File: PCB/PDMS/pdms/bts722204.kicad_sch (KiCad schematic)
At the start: 21 parts, among them IC7 BTS722204ESAXUMA1

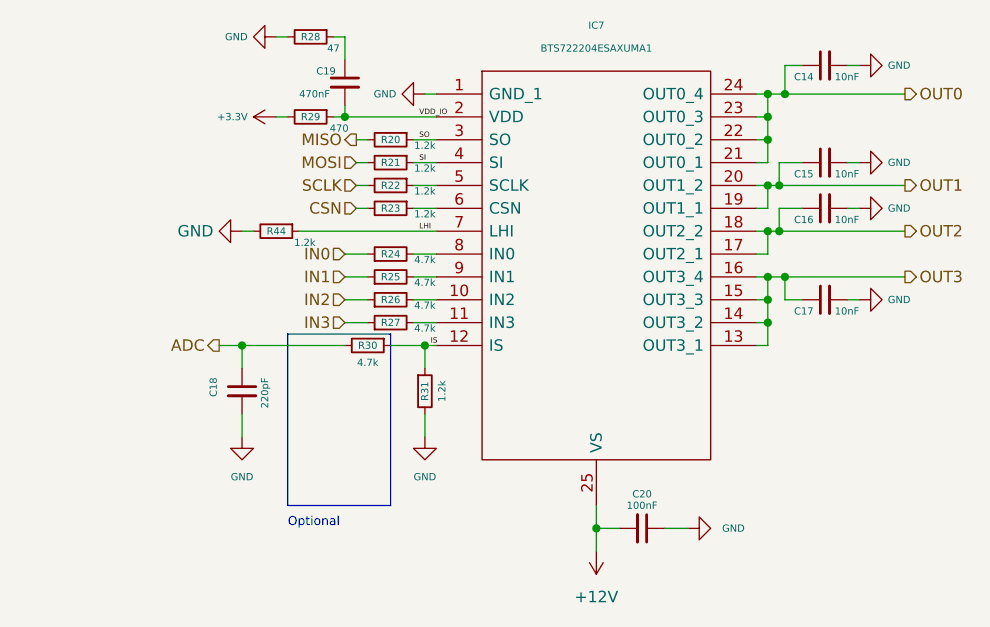
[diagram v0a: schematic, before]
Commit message: Major changes with new switch
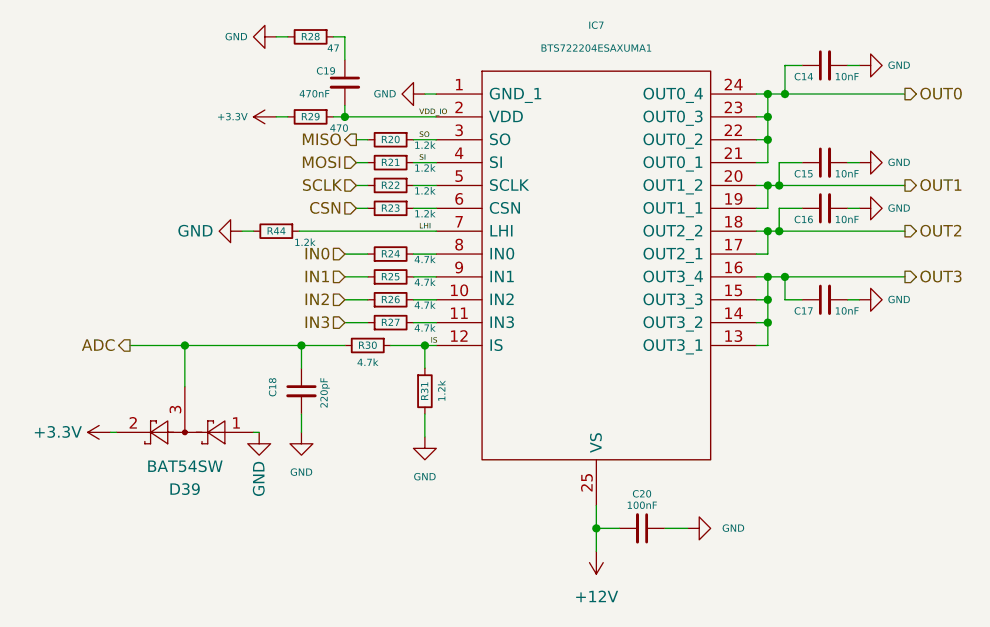
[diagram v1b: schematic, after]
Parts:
- added D39: BAT54SW, Package_TO_SOT_SMD:SOT-323_SC-70, symbol Diode:BAT54SW
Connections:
- net +3.3V: now also D39.2
- net ADC: now also D39.3
- net GND: now also D39.1
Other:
- note removed: "Optional"
- moved on the sheet: C18
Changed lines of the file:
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@@
   (junction (at 59.69 71.12) (diameter 0) (color 0 0 0 0)
   )
+  (junction (at 33.02 71.12) (diameter 0) (color 0 0 0 0)
+  )
   (junction (at 97.79 43.18) (diameter 0) (color 0 0 0 0)
   )
@@
   (junction (at 99.06 58.42) (diameter 0) (color 0 0 0 0)
   )
-  (junction (at 39.37 71.12) (diameter 0) (color 0 0 0 0)
+  (junction (at 45.974 71.12) (diameter 0) (color 0 0 0 0)
   )
   (junction (at 97.79 48.26) (diameter 0) (color 0 0 0 0)
@@
     (stroke (width 0) (type default) (color 0 0 0 0))
   )
-  (wire (pts (xy 39.37 71.12) (xy 50.8 71.12))
+  (wire (pts (xy 45.974 71.12) (xy 50.8 71.12))
     (stroke (width 0) (type default) (color 0 0 0 0))
   )
@@
     (stroke (width 0) (type default) (color 0 0 0 0))
   )
-  (polyline (pts (xy 44.45 69.85) (xy 44.45 88.9))
-    (stroke (width 0) (type default) (color 0 0 0 0))
-  )
   (wire (pts (xy 97.79 66.04) (xy 97.79 68.58))
     (stroke (width 0) (type default) (color 0 0 0 0))
@@
     (stroke (width 0) (type default) (color 0 0 0 0))
   )
-  (polyline (pts (xy 44.45 69.85) (xy 55.88 69.85))
-    (stroke (width 0) (type default) (color 0 0 0 0))
-  )
   (wire (pts (xy 50.8 66.04) (xy 53.34 66.04))
     (stroke (width 0) (type default) (color 0 0 0 0))
@@
     (stroke (width 0) (type default) (color 0 0 0 0))
   )
-  (wire (pts (xy 39.37 71.12) (xy 39.37 73.66))
+  (wire (pts (xy 45.974 71.12) (xy 45.974 73.66))
     (stroke (width 0) (type default) (color 0 0 0 0))
   )
@@
     (stroke (width 0) (type default) (color 0 0 0 0))
   )
+  (wire (pts (xy 41.275 80.772) (xy 40.64 80.772))
+    (stroke (width 0) (type default) (color 0 0 0 0))
+  )
   (wire (pts (xy 50.8 60.96) (xy 53.34 60.96))
     (stroke (width 0) (type default) (color 0 0 0 0))
@@
     (stroke (width 0) (type default) (color 0 0 0 0))
   )
-  (wire (pts (xy 36.83 71.12) (xy 39.37 71.12))
+  (wire (pts (xy 26.924 71.12) (xy 33.02 71.12))
     (stroke (width 0) (type default) (color 0 0 0 0))
   )
@@
     (stroke (width 0) (type default) (color 0 0 0 0))
   )
-  (wire (pts (xy 39.37 78.74) (xy 39.37 81.28))
+  (wire (pts (xy 45.974 78.74) (xy 45.974 80.772))
     (stroke (width 0) (type default) (color 0 0 0 0))
   )
@@
     (stroke (width 0) (type default) (color 0 0 0 0))
   )
-  (polyline (pts (xy 44.45 88.9) (xy 55.88 88.9))
-    (stroke (width 0) (type default) (color 0 0 0 0))
-  )
   (wire (pts (xy 55.88 71.12) (xy 59.69 71.12))
     (stroke (width 0) (type default) (color 0 0 0 0))
@@
     (stroke (width 0) (type default) (color 0 0 0 0))
   )
-  (polyline (pts (xy 55.88 88.9) (xy 55.88 69.85))
-    (stroke (width 0) (type default) (color 0 0 0 0))
-  )
   (wire (pts (xy 97.79 71.12) (xy 96.52 71.12))
     (stroke (width 0) (type default) (color 0 0 0 0))
   )
+  (wire (pts (xy 33.02 71.12) (xy 33.02 75.692))
+    (stroke (width 0) (type default) (color 0 0 0 0))
+  )
   (wire (pts (xy 97.79 48.26) (xy 97.79 45.72))
     (stroke (width 0) (type default) (color 0 0 0 0))
@@
     (stroke (width 0) (type default) (color 0 0 0 0))
   )
+  (wire (pts (xy 24.765 80.772) (xy 25.4 80.772))
+    (stroke (width 0) (type default) (color 0 0 0 0))
+  )
   (wire (pts (xy 59.69 78.74) (xy 59.69 81.28))
     (stroke (width 0) (type default) (color 0 0 0 0))
@@
     (stroke (width 0) (type default) (color 0 0 0 0))
   )
+  (wire (pts (xy 33.02 71.12) (xy 45.974 71.12))
+    (stroke (width 0) (type default) (color 0 0 0 0))
+  )
   (wire (pts (xy 78.74 91.44) (xy 81.28 91.44))
     (stroke (width 0) (type default) (color 0 0 0 0))
@@
   (wire (pts (xy 97.79 63.5) (xy 97.79 66.04))
     (stroke (width 0) (type default) (color 0 0 0 0))
-  )
-  (text "Optional" (at 44.45 91.44 0)
-    (effects (font (size 1 1)) (justify left bottom))
   )
   (label "IS" (at 60.325 71.12 0)
@@
     (effects (font (size 1.27 1.27)) (justify left))
   )
-  (hierarchical_label "ADC" (shape output) (at 36.83 71.12 180)
+  (hierarchical_label "ADC" (shape output) (at 26.924 71.12 180)
     (effects (font (size 1.27 1.27)) (justify right))
   )
   (hierarchical_label "IN3" (shape input) (at 50.8 68.58 180)
     (effects (font (size 1.27 1.27)) (justify right))
+  )
+  (symbol (lib_id "Diode:BAT54SW") (at 33.02 80.772 180) (unit 1)
+    (in_bom yes) (on_board yes) (fields_autoplaced)
+    (property "Reference" "D39" (id 0) (at 33.02 87.122 0))
+    (property "Value" "BAT54SW" (id 1) (at 33.02 84.582 0))
+    (property "Footprint" "Package_TO_SOT_SMD:SOT-323_SC-70" (id 2) (at 31.115 83.947 0)
+      (effects (font (size 1.27 1.27)) (justify left) hide)
+    )
+    (property "Datasheet" "https://assets.nexperia.com/documents/data-sheet/BAT54W_SER.pdf" (id 3) (at 36.068 80.772 0)
+      (effects (font (size 1.27 1.27)) hide)
+    )
+    (pin "1")
+    (pin "2")
+    (pin "3")
   )
   (symbol (lib_id "Device:R_Small") (at 55.88 68.58 90) (unit 1)
@@
     (pin "1")
   )
+  (symbol (lib_id "power:+3.3V") (at 24.765 80.772 90) (unit 1)
+    (in_bom yes) (on_board yes) (fields_autoplaced)
+    (property "Reference" "#PWR0417" (id 0) (at 28.575 80.772 0)
+      (effects (font (size 1.27 1.27)) hide)
+    )
+    (property "Value" "+3.3V" (id 1) (at 21.59 80.7721 90)
+      (effects (font (size 1.27 1.27)) (justify left))
+    )
+    (property "Footprint" "" (id 2) (at 24.765 80.772 0)
+      (effects (font (size 1.27 1.27)) hide)
+    )
+    (property "Datasheet" "" (id 3) (at 24.765 80.772 0)
+      (effects (font (size 1.27 1.27)) hide)
+    )
+    (pin "1")
+  )
   (symbol (lib_id "Device:R_Small") (at 59.69 76.2 0) (unit 1)
     (in_bom yes) (on_board yes)
@@
     (pin "2")
   )
-  (symbol (lib_id "Device:C_Small") (at 39.37 76.2 0) (unit 1)
-    (in_bom yes) (on_board yes)
-    (property "Reference" "C18" (id 0) (at 36.195 76.835 90)
-      (effects (font (size 0.8 0.8)) (justify left))
-    )
-    (property "Value" "220pF" (id 1) (at 41.91 78.105 90)
-      (effects (font (size 0.8 0.8)) (justify left))
-    )
-    (property "Footprint" "Capacitor_SMD:C_0402_1005Metric" (id 2) (at 39.37 76.2 0)
-      (effects (font (size 1.27 1.27)) hide)
-    )
-    (property "Datasheet" "~" (id 3) (at 39.37 76.2 0)
+  (symbol (lib_id "Device:C_Small") (at 45.974 76.2 0) (unit 1)
+    (in_bom yes) (on_board yes)
+    (property "Reference" "C18" (id 0) (at 42.799 76.835 90)
+      (effects (font (size 0.8 0.8)) (justify left))
+    )
+    (property "Value" "220pF" (id 1) (at 48.514 78.105 90)
+      (effects (font (size 0.8 0.8)) (justify left))
+    )
+    (property "Footprint" "Capacitor_SMD:C_0402_1005Metric" (id 2) (at 45.974 76.2 0)
+      (effects (font (size 1.27 1.27)) hide)
+    )
+    (property "Datasheet" "~" (id 3) (at 45.974 76.2 0)
       (effects (font (size 1.27 1.27)) hide)
     )
@@
     (pin "2")
   )
+  (symbol (lib_id "power:GND") (at 41.275 80.772 0) (unit 1)
+    (in_bom yes) (on_board yes) (fields_autoplaced)
+    (property "Reference" "#PWR0416" (id 0) (at 41.275 87.122 0)
+      (effects (font (size 1.27 1.27)) hide)
+    )
+    (property "Value" "GND" (id 1) (at 41.2751 83.947 90)
+      (effects (font (size 1.27 1.27)) (justify right))
+    )
+    (property "Footprint" "" (id 2) (at 41.275 80.772 0)
+      (effects (font (size 1.27 1.27)) hide)
+    )
+    (property "Datasheet" "" (id 3) (at 41.275 80.772 0)
+      (effects (font (size 1.27 1.27)) hide)
+    )
+    (pin "1")
+  )
   (symbol (lib_id "Device:R_Small") (at 55.88 55.88 270) (unit 1)
     (in_bom yes) (on_board yes)
@@
     (pin "1")
   )
-  (symbol (lib_id "power:GND") (at 39.37 81.28 0) (unit 1)
-    (in_bom yes) (on_board yes) (fields_autoplaced)
-    (property "Reference" "#PWR0131" (id 0) (at 39.37 87.63 0)
+  (symbol (lib_id "power:GND") (at 45.974 80.772 0) (unit 1)
+    (in_bom yes) (on_board yes) (fields_autoplaced)
+    (property "Reference" "#PWR0131" (id 0) (at 45.974 87.122 0)
       (effects (font (size 0.8 0.8)) hide)
     )
-    (property "Value" "GND" (id 1) (at 39.37 85.725 0)
-      (effects (font (size 0.8 0.8)))
-    )
-    (property "Footprint" "" (id 2) (at 39.37 81.28 0)
-      (effects (font (size 1.27 1.27)) hide)
-    )
-    (property "Datasheet" "" (id 3) (at 39.37 81.28 0)
-      (effects (font (size 1.27 1.27)) hide)
-    )
+    (property "Value" "GND" (id 1) (at 45.974 85.217 0)
+      (effects (font (size 0.8 0.8)))
+    )
+    (property "Footprint" "" (id 2) (at 45.974 80.772 0)
+      (effects (font (size 1.27 1.27)) hide)
+    )
+    (property "Datasheet" "" (id 3) (at 45.974 80.772 0)
+      (effects (font (size 1.27 1.27)) hide)
+    )
